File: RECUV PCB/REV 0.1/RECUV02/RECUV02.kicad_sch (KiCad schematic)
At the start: 64 parts, among them P1 VEXT, P2 VOLTAGE, P3 CURRENT, Q1 MMBT2222ALT1, Q2 MMBT2222ALT1, U1 ESP32-S3-WROOM-1, U2 CH340C, U3 A1117-3.3, U4 RESET, U5 BOOT, U6 ACS712ELCTR-20A-T

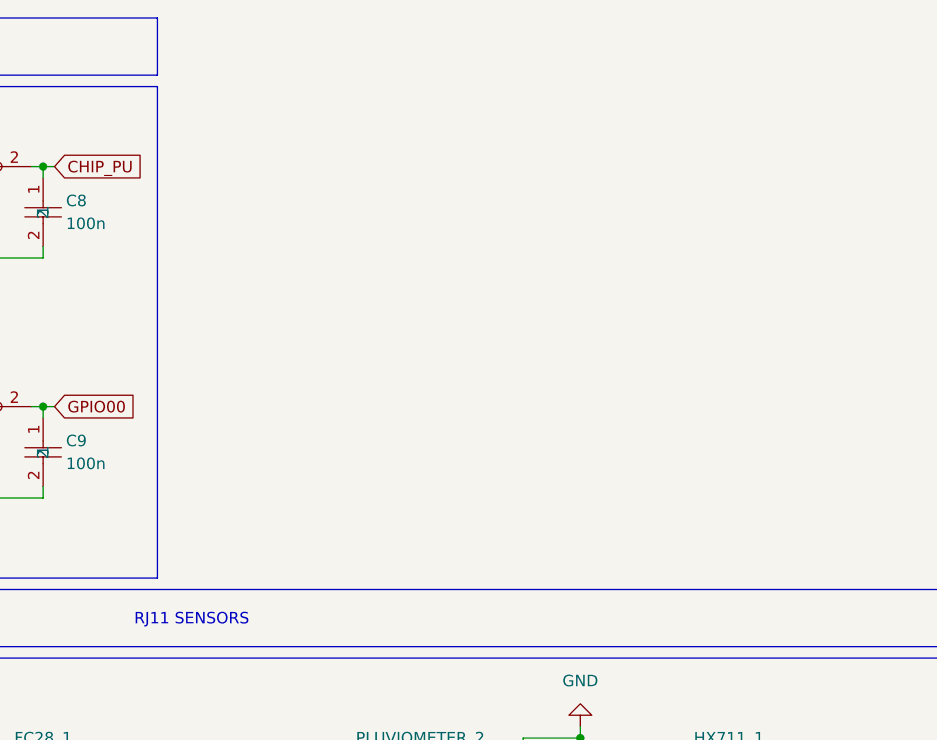
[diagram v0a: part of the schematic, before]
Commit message: Finished all PCB sections
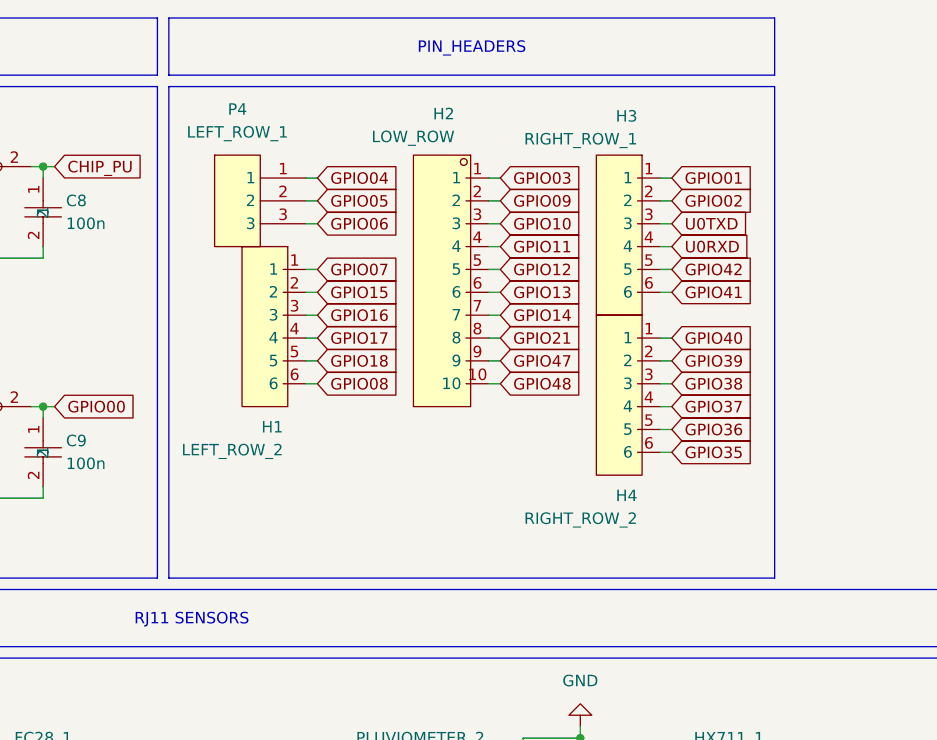
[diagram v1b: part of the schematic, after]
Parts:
- added H1: LEFT_ROW_2, EasyEDA:HDR-TH_6P-P2.54-V-M-1, symbol EasyEDA:Header-Male-2.54_1x6
- added H2: LOW_ROW, EasyEDA:HDR-TH_10P-P2.54-V-M-1, symbol EasyEDA:Header-Male-2.54_1x10
- added H3: RIGHT_ROW_1, EasyEDA:HDR-TH_6P-P2.54-V-M-1, symbol EasyEDA:Header-Male-2.54_1x6
- added H4: RIGHT_ROW_2, EasyEDA:HDR-TH_6P-P2.54-V-M-1, symbol EasyEDA:Header-Male-2.54_1x6
- added P4: LEFT_ROW_1, EasyEDA:HDR-TH_3P-P1.27-V-M-1, symbol EasyEDA:1.27mm_1*3p
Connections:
- net GPIO01: now also H3.1
- net GPIO02: now also H3.2
- net GPIO03: now also H2.1
- net GPIO04: now also P4.1
- net GPIO05: now also P4.2
- net GPIO06: now also P4.3
- net GPIO07: now also H1.1
- net GPIO08: now also H1.6
- net GPIO09: now also H2.2
- net GPIO10: now also H2.3
- net GPIO11: now also H2.4
- net GPIO12: now also H2.5
- net GPIO13: now also H2.6
- net GPIO14: now also H2.7
- net GPIO15: now also H1.2
- net GPIO16: now also H1.3
- net GPIO17: now also H1.4
- net GPIO18: now also H1.5
- net GPIO21: now also H2.8
- net GPIO35: now also H4.6
- net GPIO36: now also H4.5
- net GPIO37: now also H4.4
- net GPIO38: now also H4.3
- net GPIO39: now also H4.2
- net GPIO40: now also H4.1
- net GPIO41: now also H3.6
- net GPIO42: now also H3.5
- net GPIO47: now also H2.9
- net GPIO48: now also H2.10
- net U0RXD: now also H3.4
- net U0TXD: now also H3.3
